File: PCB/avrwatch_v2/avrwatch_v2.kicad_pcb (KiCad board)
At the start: 2 copper layers, 29.2 x 29.2 mm, 9 parts, among them J1 ICP, SW1 SW_Push, SW2 SW_Push, U1 ATmega328P-AU, U2 KCSA02-105, Y1 ABS07-120-32.768KHZ-T

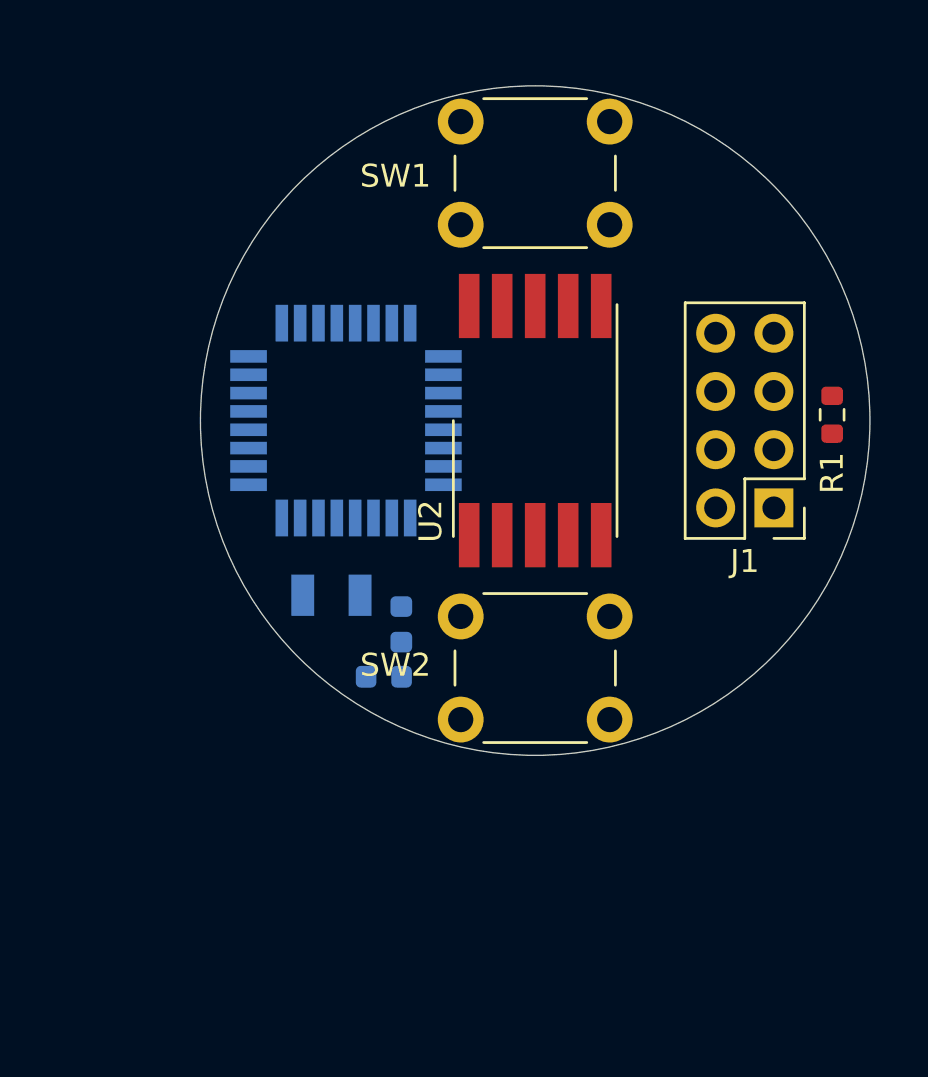
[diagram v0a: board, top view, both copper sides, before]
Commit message: finishing the pcb
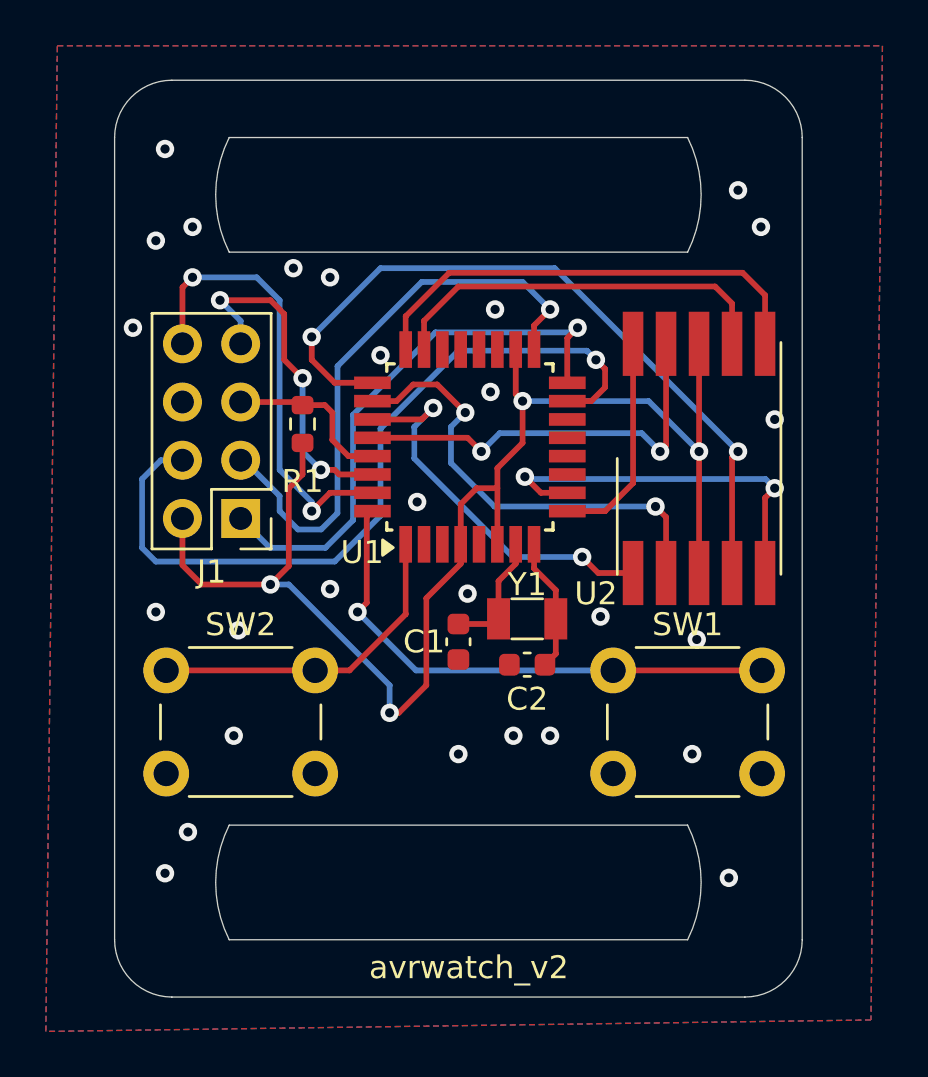
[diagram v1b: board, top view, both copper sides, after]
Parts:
- C1, C2, U1, Y1: moved to F.Cu
- SW1, SW2: footprint MoireLabs:SW_PUSH_6mm_H9.5mm_center -> QuorumPrecision:SW_PUSH_6mm_H9.5mm_center
- moved SW1 24.9 mm to (140.0, 83.0)
- moved J1 23.3 mm to (120.5, 74.1)
- moved R1 23.1 mm to (123.2, 70.0)
- moved SW2 13.1 mm to (120.5, 83.0)
- moved Y1 8.60 mm to (133.0, 78.5), turned to 180 degrees
- moved U2 7.34 mm to (140.5, 71.5)
- moved C2 6.28 mm to (133.0, 80.5), turned to 0 degrees
- moved U1 5.53 mm to (130.5, 71.0)
- moved C1 2.61 mm to (130.0, 79.5)
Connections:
- J1 pad 1: (no net) -> /MISO
- J1 pad 3: (no net) -> /SCK
- J1 pad 4: (no net) -> /MOSI
- J1 pad 7: (no net) -> /RX
- J1 pad 8: (no net) -> /TX
- U1 pad 11: (no net) -> unconnected-(U1-PD7-Pad11)
- U1 pad 12: (no net) -> unconnected-(U1-PB0-Pad12)
- U1 pad 13: (no net) -> unconnected-(U1-PB1-Pad13)
- U1 pad 14: (no net) -> unconnected-(U1-PB2-Pad14)
- U1 pad 15: (no net) -> /MOSI
- U1 pad 16: (no net) -> /MISO
- U1 pad 17: (no net) -> /SCK
- U1 pad 19: (no net) -> unconnected-(U1-ADC6-Pad19)
- U1 pad 2: (no net) -> unconnected-(U1-PD4-Pad2)
- U1 pad 20: (no net) -> unconnected-(U1-AREF-Pad20)
- U1 pad 22: (no net) -> unconnected-(U1-ADC7-Pad22)
- U1 pad 30: (no net) -> /RX
- U1 pad 31: (no net) -> /TX
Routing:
- net VCC: track 0.00 -> 61.4 mm, vias 0 -> 4
- net /MOSI: track 0.00 -> 34.6 mm, vias 0 -> 1
- net Net-(U1-PC2): track 0.00 -> 32.6 mm, vias 0 -> 2
- net /SCK: track 0.00 -> 25.9 mm, vias 0 -> 1
- net /MISO: track 0.00 -> 24.5 mm, vias 0 -> 1
- net Net-(U1-PD2): track 0.00 -> 23.4 mm, vias 0 -> 1
- net Net-(U1-PC1): track 0.00 -> 20.4 mm
- net Net-(U1-PC3): track 0.00 -> 20.1 mm, vias 0 -> 2
- net /TX: track 0.00 -> 20.1 mm, vias 0 -> 2
- net Net-(U1-PC5): track 0.00 -> 18.3 mm, vias 0 -> 2
- net Net-(U1-PC0): track 0.00 -> 17.4 mm
- net Net-(U1-PD6): track 0.00 -> 17.1 mm, vias 0 -> 2
- net Net-(U1-PC4): track 0.00 -> 17.0 mm, vias 0 -> 2
- net /RX: track 0.00 -> 15.1 mm, vias 0 -> 3
- net Net-(U1-PD3): track 0.00 -> 14.5 mm
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- added copper zone on B.Cu, net GND
- added copper zone on F.Cu, net GND
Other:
- board size 29.2 x 29.2 mm -> 30 x 40 mm
- net class Default removed
- board text added: "avrwatch_v2"
